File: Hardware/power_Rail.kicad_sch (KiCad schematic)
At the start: 13 parts

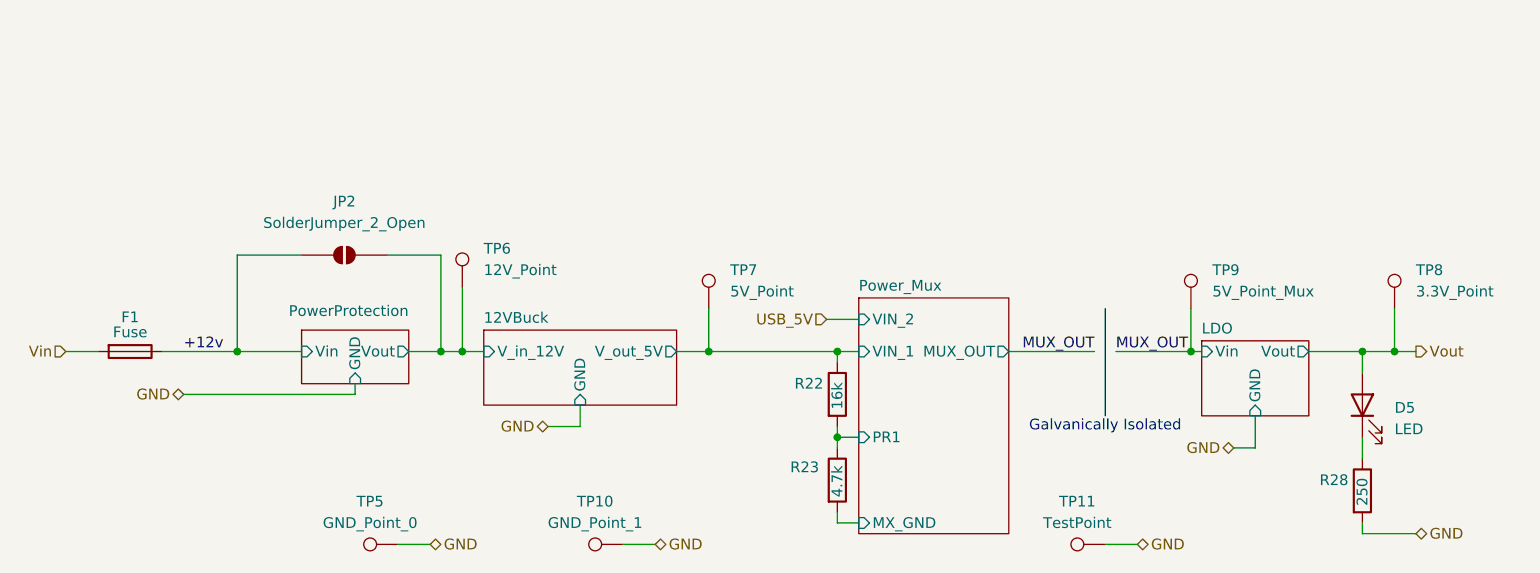
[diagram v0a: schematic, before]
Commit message: Final Review Ready
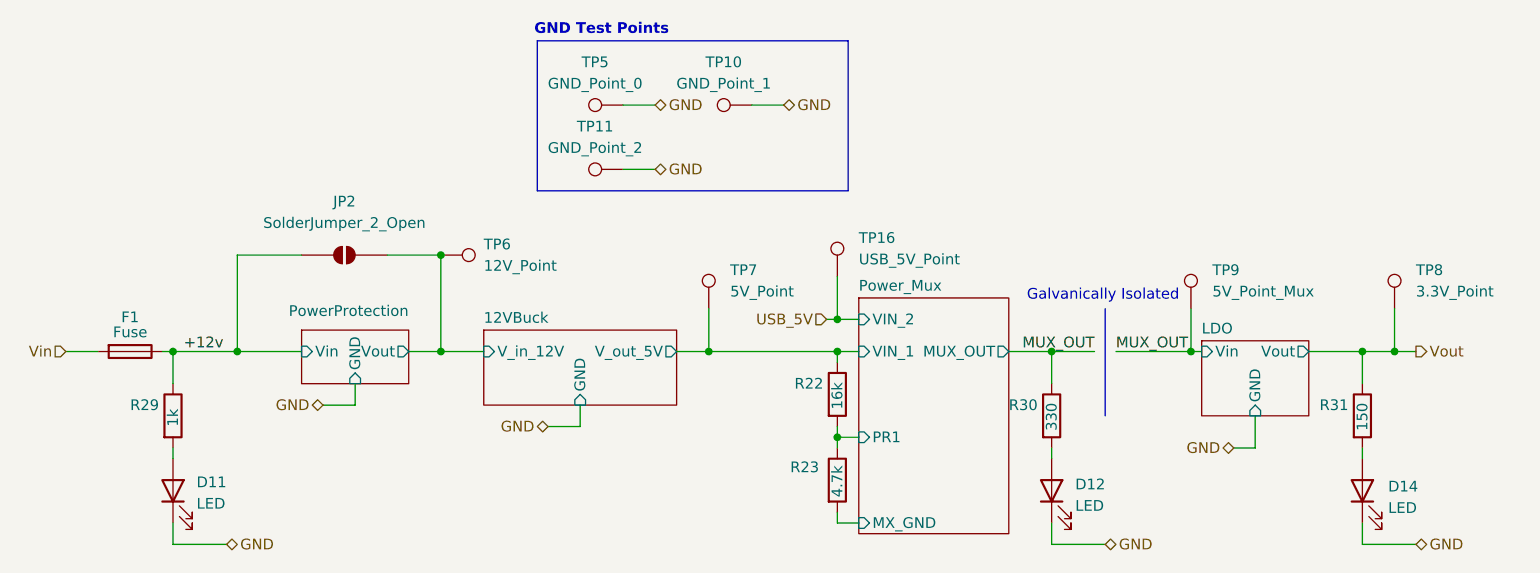
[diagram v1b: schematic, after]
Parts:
- removed D5: LED, LED_SMD:LED_0603_1608Metric, symbol lhrs_misc:Blue_LED
- removed R28: 250, Package_TO_SOT_SMD:SOT-23, symbol Device:R
- added D11, D12, D14: LED, LED_SMD:LED_0603_1608Metric_Pad1.05x0.95mm_HandSolder, symbol lhrs_misc:Blue_LED
- added R29: 1k, Package_TO_SOT_SMD:SOT-23, symbol Device:R
- added R30: 330, Package_TO_SOT_SMD:SOT-23, symbol Device:R
- added R31: 150, Package_TO_SOT_SMD:SOT-23, symbol Device:R
- added TP16: USB_5V_Point, LHRS_Connectors:Molex_Nano-Fit_105310-xx10_2x05_P2.50mm_Vertical, symbol Connector:TestPoint
- TP11: value TestPoint -> GND_Point_2
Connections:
- net +12v: now also R29.1
- net GND: now also D11.1 (K), D12.1 (K), D14.1 (K)
- net MUX_OUT: now also R30.1
- net USB_5V: now also TP16.1
- net Vout: now also R31.1
- new net: D11.2 (A), R29.2
- new net: D14.2 (A), R31.2
- new net: D12.2 (A), R30.2
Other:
- note added: "GND Test Points"
- moved on the sheet: TP10, TP11, TP5, TP6
